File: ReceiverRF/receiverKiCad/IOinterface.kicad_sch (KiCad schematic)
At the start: 20 parts, among them Q1 MMBT3904, SW1 SW_Push, SW2 SW_Push, SW3 SW_Push, SW4 SW_Push

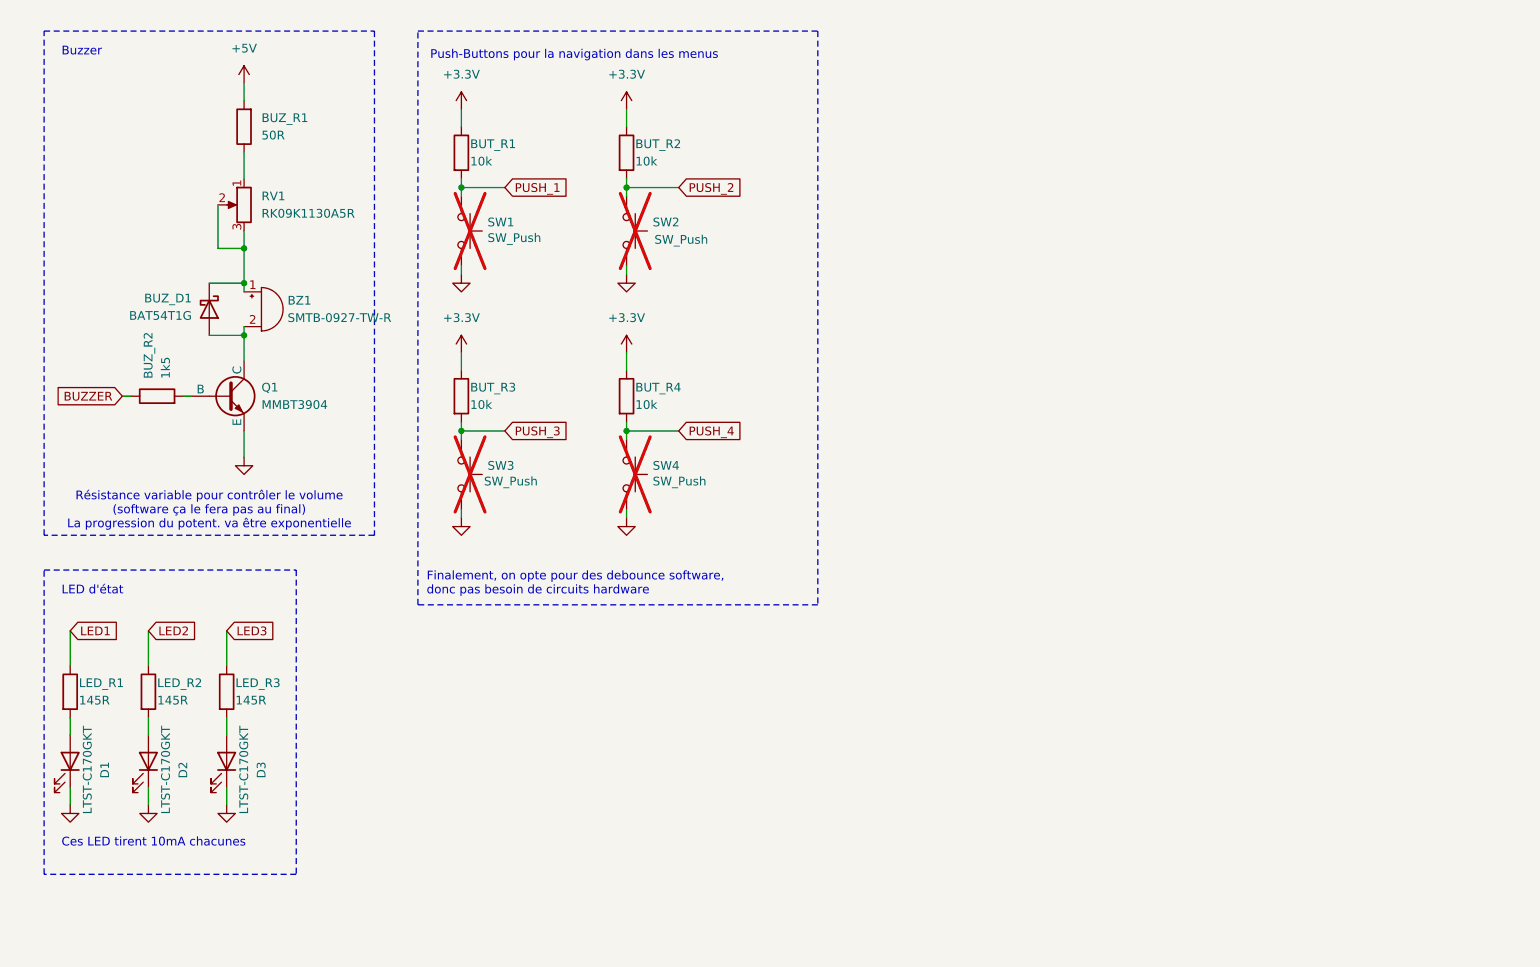
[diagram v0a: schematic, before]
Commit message: ideFIX v2 fix schematic, layout
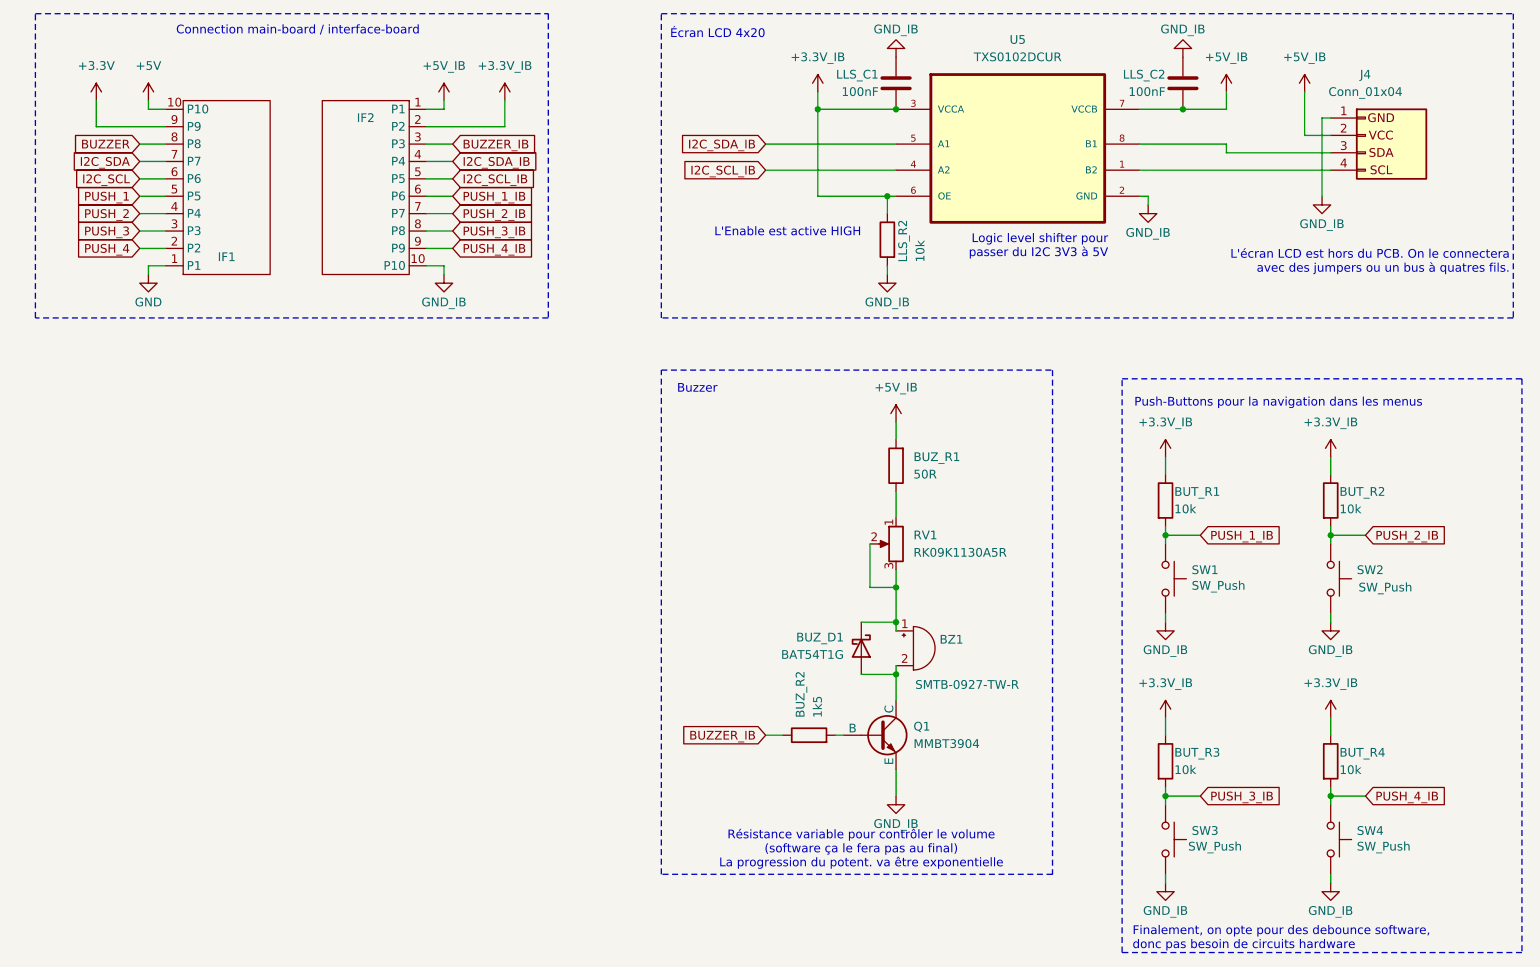
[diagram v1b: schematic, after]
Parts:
- removed D1, D2, D3: LTST-C170GKT, Footprints:LTST-C170GKT, symbol Device:LED
- removed LED_R1, LED_R2, LED_R3: 145R, Resistor_SMD:R_1206_3216Metric, symbol Device:R
- added IF1, IF2: ~, Footprints:CONN10_530481010_MOL, symbol Symboles:INTERFACE_BOARD
- added J4: Conn_01x04, Connector_PinHeader_2.54mm:PinHeader_1x04_P2.54mm_Vertical, symbol Connector_Generic:Conn_01x04
- added LLS_C1, LLS_C2: 100nF, Capacitor_SMD:C_1206_3216Metric, symbol Device:C
- added LLS_R2: 10k, Resistor_SMD:R_1206_3216Metric, symbol Device:R
- added U5: TXS0102DCUR, Footprints:SOP50P310X90-8N, symbol Symboles:TXS0102DCUR
- SW1, SW2, SW3, SW4: now fitted
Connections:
- net +3.3V: now also IF1.9 (P9); no longer BUT_R1.1, BUT_R2.1, BUT_R3.1, BUT_R4.1
- net +5V: now also IF1.10 (P10); no longer BUZ_R1.2
- net BUZZER: now also IF1.8 (P8); no longer BUZ_R2.1
- net GND: now also IF1.1 (P1); no longer Q1.3 (E), SW1.2, SW2.2, SW3.2, SW4.2
- net PUSH_1: now also IF1.5 (P5); no longer BUT_R1.2, SW1.1
- net PUSH_2: now also IF1.4 (P4); no longer BUT_R2.2, SW2.1
- net PUSH_3: now also IF1.3 (P3); no longer BUT_R3.2, SW3.1
- net PUSH_4: now also IF1.2 (P2); no longer BUT_R4.2, SW4.1
- new net: J4.3 (SDA), U5.8 (B1)
- new net: J4.4 (SCL), U5.1 (B2)
- new net +3.3V_IB: BUT_R1.1, BUT_R2.1, BUT_R3.1, BUT_R4.1, IF2.2 (P2), LLS_C1.2, LLS_R2.1, U5.3 (VCCA), U5.6 (OE)
- new net +5V_IB: BUZ_R1.2, IF2.1 (P1), J4.2 (VCC), LLS_C2.2, U5.7 (VCCB)
- new net BUZZER_IB: BUZ_R2.1, IF2.3 (P3)
- new net GND_IB: IF2.10 (P10), J4.1 (GND), LLS_C1.1, LLS_C2.1, LLS_R2.2, Q1.3 (E), SW1.2, SW2.2, SW3.2, SW4.2, U5.2 (GND)
- new net I2C_SCL: IF1.6 (P6)
- new net I2C_SCL_IB: IF2.5 (P5), U5.4 (A2)
- new net I2C_SDA: IF1.7 (P7)
- new net I2C_SDA_IB: IF2.4 (P4), U5.5 (A1)
- new net PUSH_1_IB: BUT_R1.2, IF2.6 (P6), SW1.1
- new net PUSH_2_IB: BUT_R2.2, IF2.7 (P7), SW2.1
- new net PUSH_3_IB: BUT_R3.2, IF2.8 (P8), SW3.1
- new net PUSH_4_IB: BUT_R4.2, IF2.9 (P9), SW4.1
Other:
- note added: "Connection main-board / interface-board"
- note added: "L'Enable est active HIGH"
- note added: "L'écran LCD est hors du PCB. On le connectera avec des jumpers ou un bus à quatres fils."
- note added: "Logic level shifter pour passer du I2C 3V3 à 5V"
- note added: "Écran LCD 4x20"
- note removed: "Ces LED tirent 10mA chacunes"
- note removed: "LED d'état"
- moved on the sheet: BUT_R1, BUT_R2, BUT_R3, BUT_R4, BUZ_D1, BUZ_R1, BUZ_R2, BZ1, Q1, RV1

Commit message: revision schematic before tracing
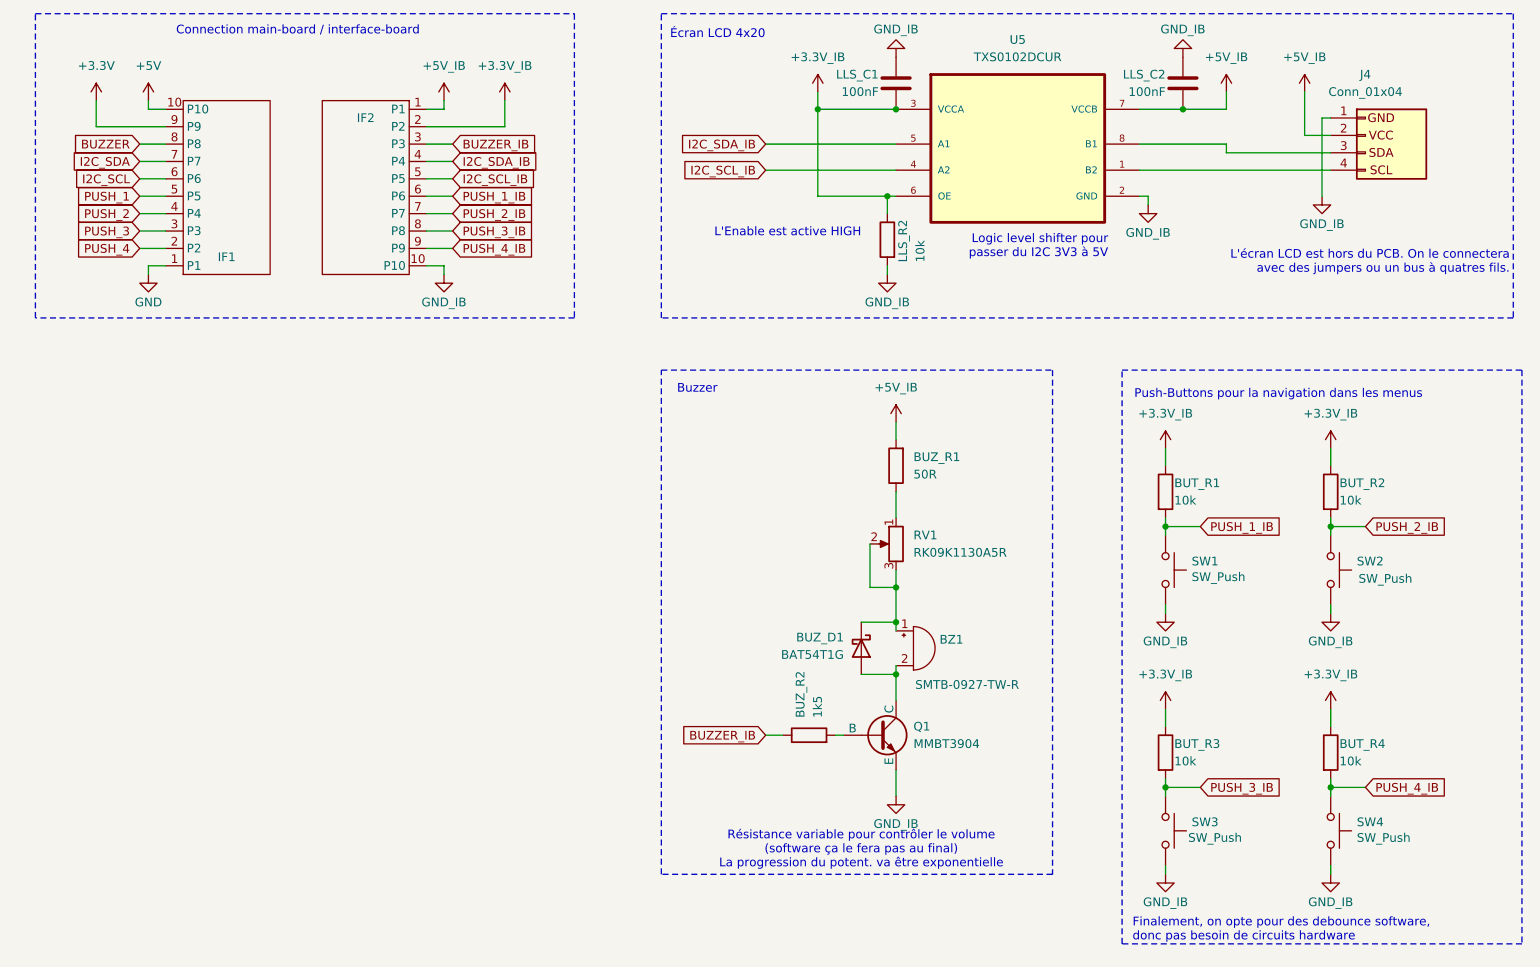
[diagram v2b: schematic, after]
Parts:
- SW1, SW2, SW3, SW4: Digikey (none) -> EG1862-ND
- U5: Digikey (none) -> 296-21931-2-ND
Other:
- company: (none) -> GAUL
- title: (none) -> IdeFIX
- moved on the sheet: BUT_R1, BUT_R2, BUT_R3, BUT_R4, SW1, SW2, SW3, SW4
